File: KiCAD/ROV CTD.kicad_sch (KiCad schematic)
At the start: 41 parts, among them J1 Conn_Coaxial, J13 Head Connector, J14 Head Connector, J15 Conn_01x07_Pin, J6 Main In, M1 EZO-EC, M2 MS5803-14BA, U2 ATtiny1614-Arduino, U3 AP63205WU, U6 MAX3072E

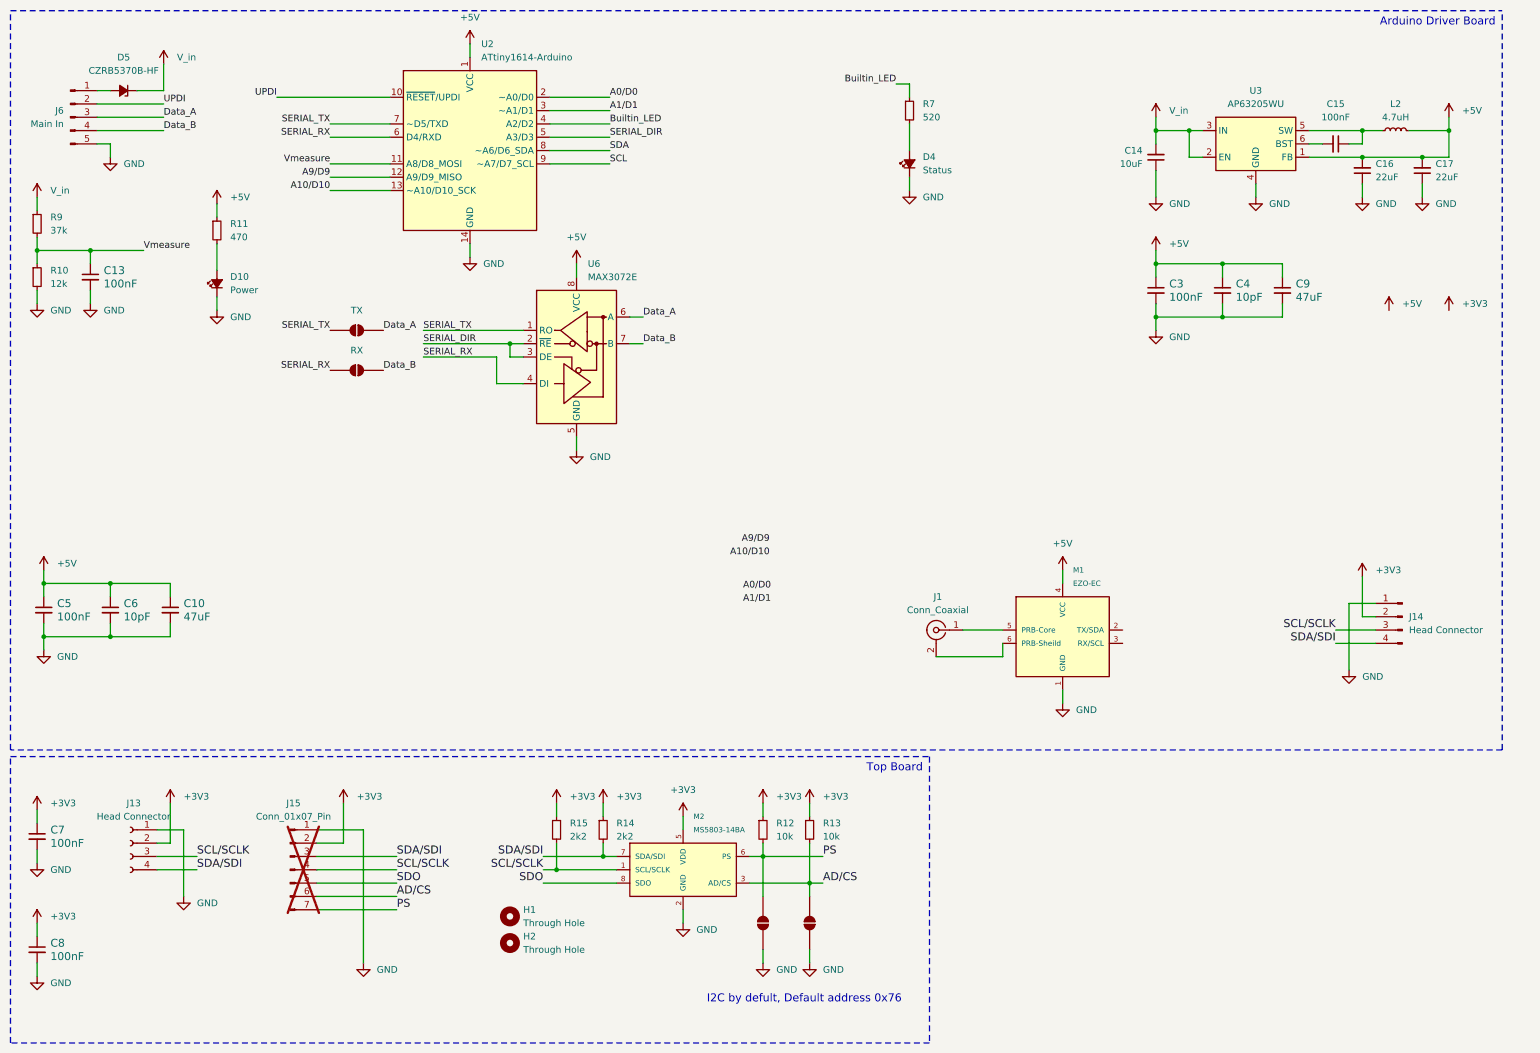
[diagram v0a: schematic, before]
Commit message: .
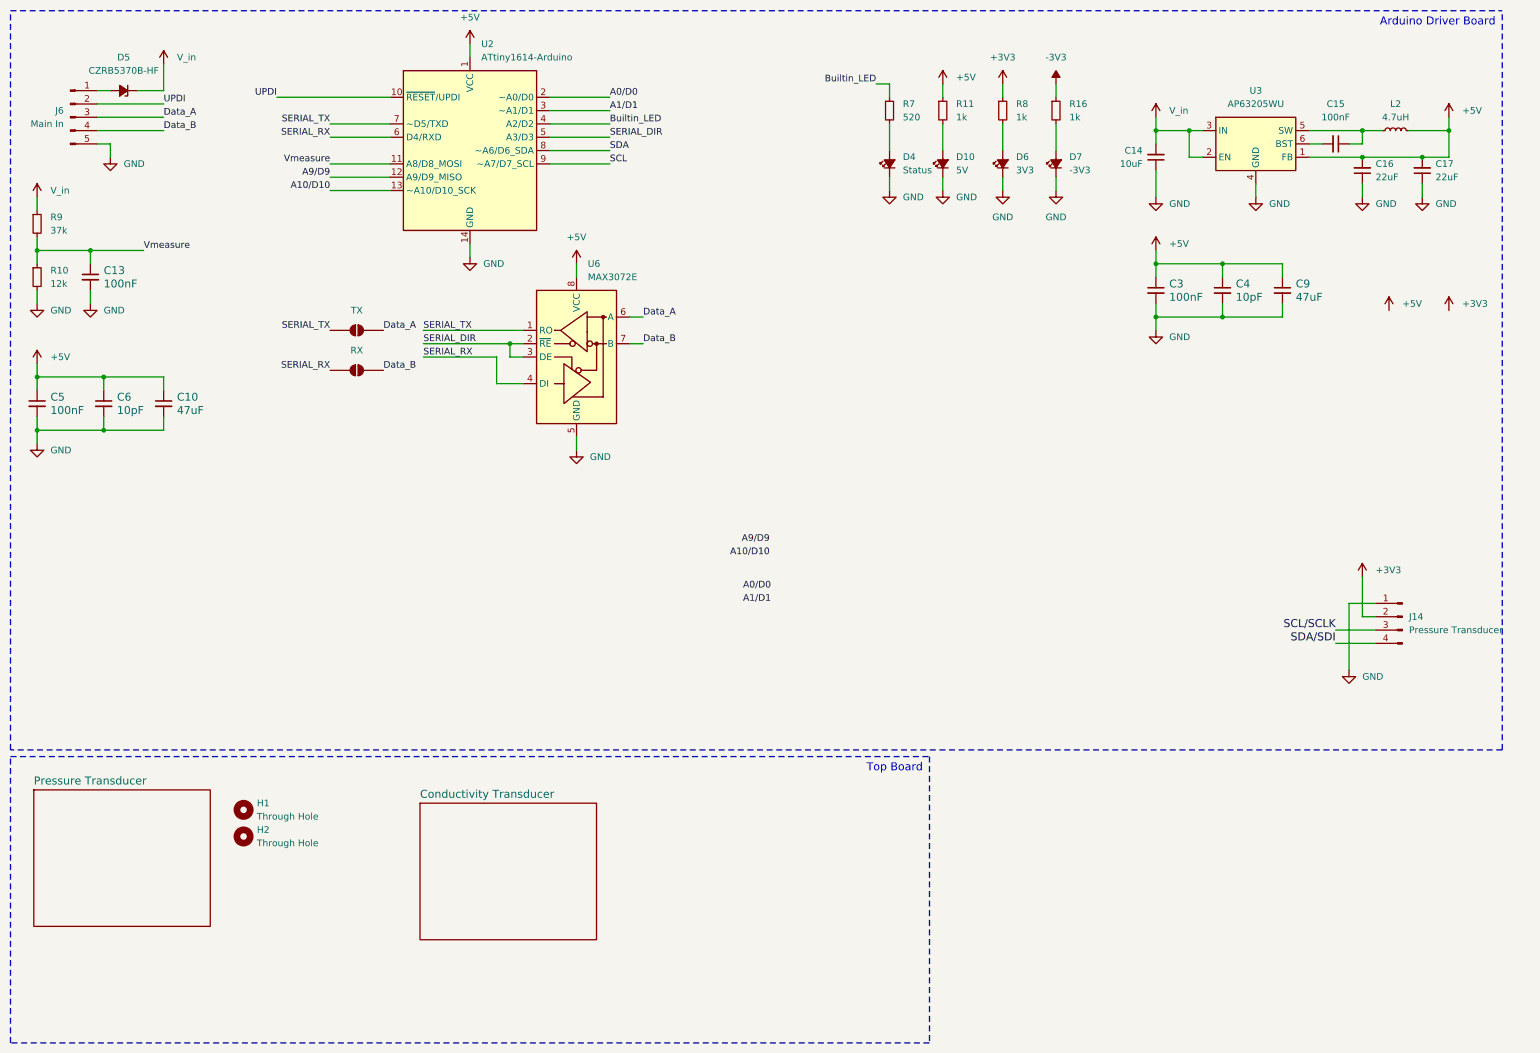
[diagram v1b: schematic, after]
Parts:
- removed C7, C8: 100nF, Capacitor_SMD:C_0805_2012Metric_Pad1.18x1.45mm_HandSolder, symbol Device:C_Small
- removed J1: Conn_Coaxial, Connector_Coaxial:BNC_TEConnectivity_1478204_Vertical, symbol Connector:Conn_Coaxial
- removed J13: Head Connector, Connector_PinSocket_2.54mm:PinSocket_1x04_P2.54mm_Vertical, symbol Connector:Conn_01x04_Socket
- removed J15: Conn_01x07_Pin, Connector_PinSocket_2.54mm:PinSocket_1x07_P2.54mm_Vertical, symbol Connector:Conn_01x07_Pin
- removed JP3, JP4: RX, Jumper:SolderJumper-2_P1.3mm_Open_TrianglePad1.0x1.5mm, symbol Jumper:SolderJumper_2_Open
- removed M1: EZO-EC, KiCad Footprints:EZO_Conductivity_Module, symbol KiCad Symbols:EZO-EC
- removed M2: MS5803-14BA, KiCad Footprints:MS5803-14BA, symbol KiCad Symbols:MS5803-14BA
- removed R12, R13: 10k, Resistor_SMD:R_0805_2012Metric_Pad1.20x1.40mm_HandSolder, symbol Device:R_Small
- removed R14, R15: 2k2, Resistor_SMD:R_0805_2012Metric_Pad1.20x1.40mm_HandSolder, symbol Device:R_Small
- added D6: 3V3, LED_SMD:LED_0805_2012Metric_Pad1.15x1.40mm_HandSolder, symbol Device:LED_Small_Filled
- added D7: -3V3, LED_SMD:LED_0805_2012Metric_Pad1.15x1.40mm_HandSolder, symbol Device:LED_Small_Filled
- added R16, R8: 1k, Resistor_SMD:R_0805_2012Metric_Pad1.20x1.40mm_HandSolder, symbol Device:R_Small
- D10: value Power -> 5V
- J14: value Head Connector -> Pressure Transducer
- R11: value 470 -> 1k
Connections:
- net +3V3: now also R8.1
- net GND: now also D6.1 (K), D7.1 (K)
- new net: D7.2 (A), R16.2
- new net: D6.2 (A), R8.2
- new net -3V3: R16.1
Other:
- added sheet Conductivity Transducer (Conductivity Transducer.kicad_sch)
- added sheet Pressure Transducer (Pressure Transducer.kicad_sch)
- note removed: "I2C by defult, Default address 0x76"
- moved on the sheet: C10, C5, C6, D10, D4, R11, R7
